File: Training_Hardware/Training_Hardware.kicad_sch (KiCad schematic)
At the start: 4 parts

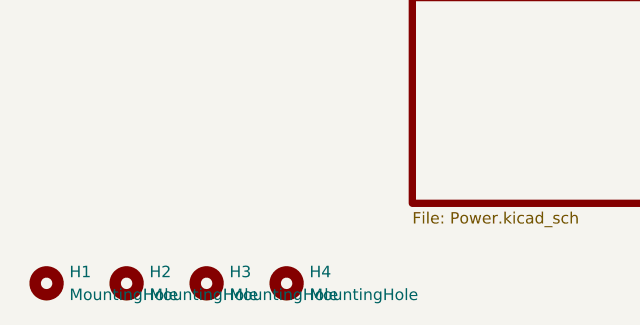
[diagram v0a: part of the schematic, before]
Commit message: PCB edits
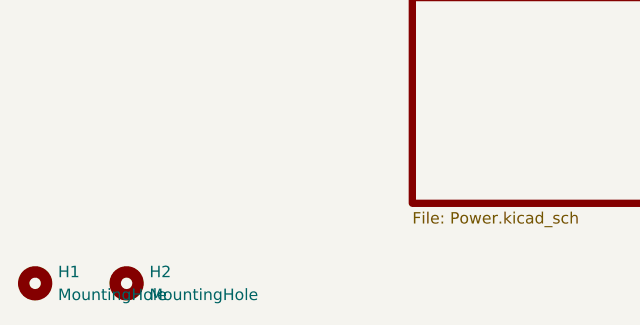
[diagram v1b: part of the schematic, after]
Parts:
- removed H3, H4: MountingHole, MRDT_Drill_Holes:4_40_Hole_Corner, symbol Mechanical:MountingHole
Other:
- moved on the sheet: H1
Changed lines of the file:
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@@
 	(symbol
 		(lib_id "Mechanical:MountingHole")
-		(at 163.83 116.84 0)
+		(at 162.56 116.84 0)
 		(unit 1)
 		(exclude_from_sim no)
@@
 		(fields_autoplaced yes)
 		(property "Reference" "H1"
-			(at 166.37 115.5699 0)
+			(at 165.1 115.5699 0)
 			(effects
 				(font
@@
 		)
 		(property "Value" "MountingHole"
-			(at 166.37 118.1099 0)
+			(at 165.1 118.1099 0)
 			(effects
 				(font
@@
 		)
 		(property "Footprint" "MRDT_Drill_Holes:4_40_Hole_Corner"
-			(at 163.83 116.84 0)
+			(at 162.56 116.84 0)
 			(effects
 				(font
@@
 		)
 		(property "Datasheet" "~"
-			(at 163.83 116.84 0)
+			(at 162.56 116.84 0)
 			(effects
 				(font
@@
 		)
 		(property "Description" "Mounting Hole without connection"
-			(at 163.83 116.84 0)
+			(at 162.56 116.84 0)
 			(effects
 				(font
@@
 					(unit 1)
 				)
-			)
-		)
-	)
-	(symbol
-		(lib_id "Mechanical:MountingHole")
-		(at 190.5 116.84 0)
-		(unit 1)
-		(exclude_from_sim no)
-		(in_bom no)
-		(on_board yes)
-		(dnp no)
-		(fields_autoplaced yes)
-		(property "Reference" "H4"
-			(at 193.04 115.5699 0)
-			(effects
-				(font
-					(size 1.27 1.27)
-				)
-				(justify left)
-			)
-		)
-		(property "Value" "MountingHole"
-			(at 193.04 118.1099 0)
-			(effects
-				(font
-					(size 1.27 1.27)
-				)
-				(justify left)
-			)
-		)
-		(property "Footprint" "MRDT_Drill_Holes:4_40_Hole_Corner"
-			(at 190.5 116.84 0)
-			(effects
-				(font
-					(size 1.27 1.27)
-				)
-				(hide yes)
-			)
-		)
-		(property "Datasheet" "~"
-			(at 190.5 116.84 0)
-			(effects
-				(font
-					(size 1.27 1.27)
-				)
-				(hide yes)
-			)
-		)
-		(property "Description" "Mounting Hole without connection"
-			(at 190.5 116.84 0)
-			(effects
-				(font
-					(size 1.27 1.27)
-				)
-				(hide yes)
-			)
-		)
-		(instances
-			(project "Training_Hardware"
-				(path "/11bb8091-1487-4100-afd2-5aa288c40d4f"
-					(reference "H4")
-					(unit 1)
-				)
-			)
-		)
-	)
-	(symbol
-		(lib_id "Mechanical:MountingHole")
-		(at 181.61 116.84 0)
-		(unit 1)
-		(exclude_from_sim no)
-		(in_bom no)
-		(on_board yes)
-		(dnp no)
-		(fields_autoplaced yes)
-		(property "Reference" "H3"
-			(at 184.15 115.5699 0)
-			(effects
-				(font
-					(size 1.27 1.27)
-				)
-				(justify left)
-			)
-		)
-		(property "Value" "MountingHole"
-			(at 184.15 118.1099 0)
-			(effects
-				(font
-					(size 1.27 1.27)
-				)
-				(justify left)
-			)
-		)
-		(property "Footprint" "MRDT_Drill_Holes:4_40_Hole_Corner"
-			(at 181.61 116.84 0)
-			(effects
-				(font
-					(size 1.27 1.27)
-				)
-				(hide yes)
-			)
-		)
-		(property "Datasheet" "~"
-			(at 181.61 116.84 0)
-			(effects
-				(font
-					(size 1.27 1.27)
-				)
-				(hide yes)
-			)
-		)
-		(property "Description" "Mounting Hole without connection"
-			(at 181.61 116.84 0)
-			(effects
-				(font
-					(size 1.27 1.27)
-				)
-				(hide yes)
-			)
-		)
-		(instances
-			(project "Training_Hardware"
-				(path "/11bb8091-1487-4100-afd2-5aa288c40d4f"
-					(reference "H3")
-					(unit 1)
-				)
